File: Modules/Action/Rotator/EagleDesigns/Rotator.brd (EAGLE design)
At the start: 100 x 80 mm, 9 parts, among them U2 ATMEGA328P_TQFP

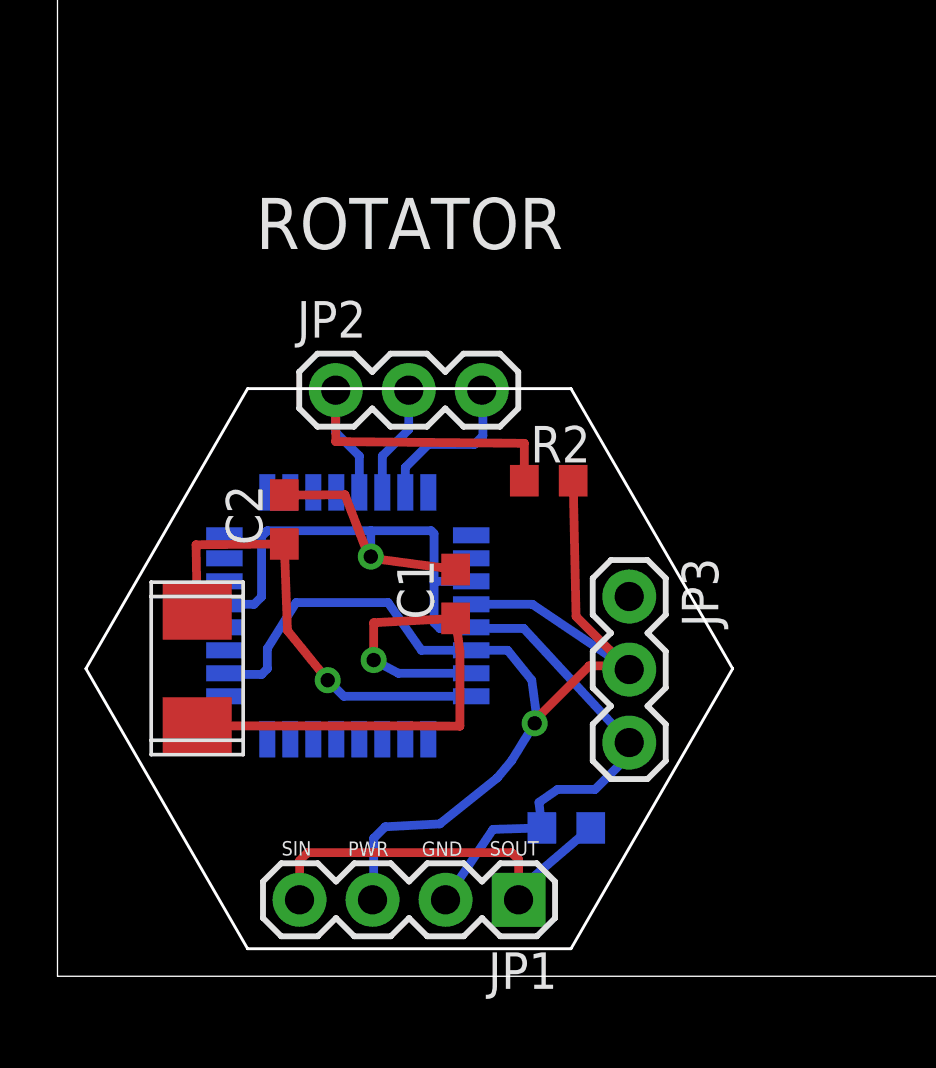
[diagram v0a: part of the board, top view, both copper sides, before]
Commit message: Revert "Merge branch 'version-1.2'"
This reverts commit 982d9c85d5bd00c48b539e840003de48d3cf178d, reversing
changes made to b3895ae538c161df72313035d3e956c7a5ec4dbc.
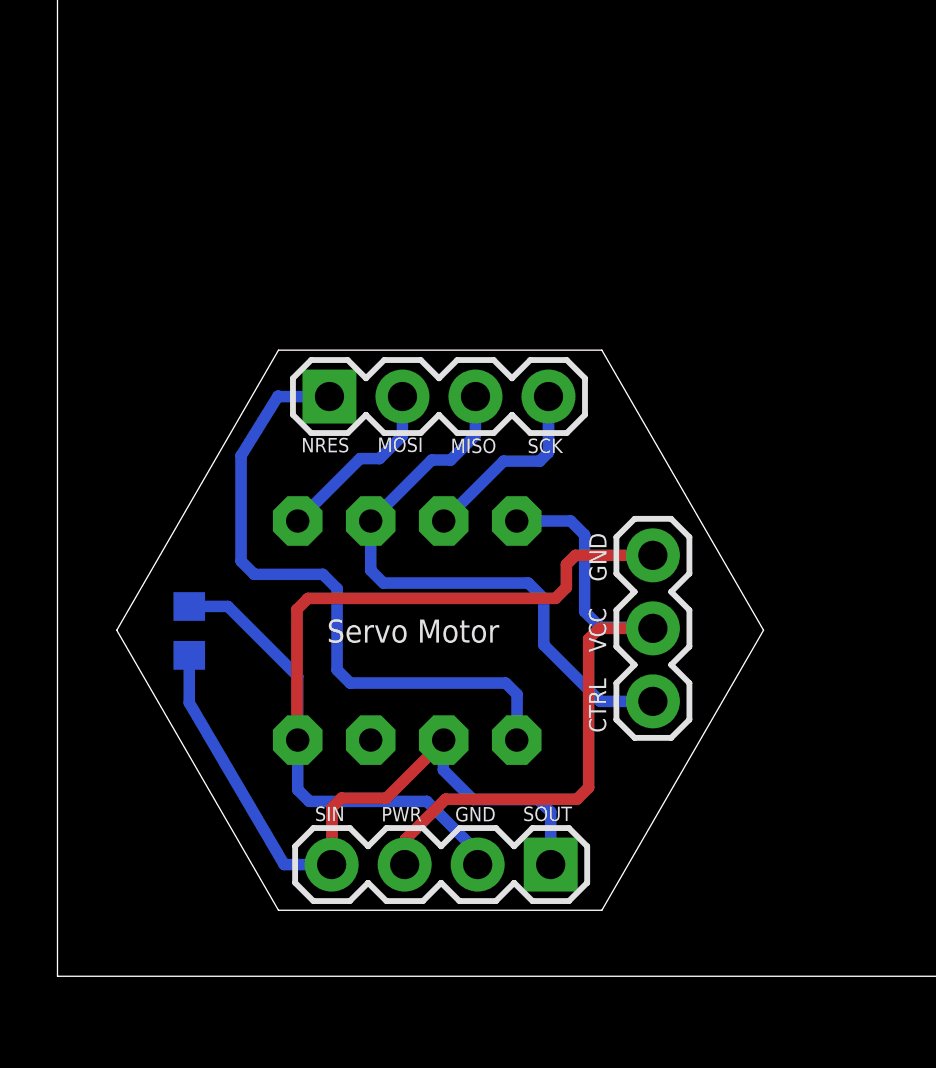
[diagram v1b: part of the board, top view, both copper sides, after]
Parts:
- removed C1, C2: 22pF, adafruit:C0603
- removed R2: 10K, resistor:R0603
- removed U$2: NX503, MakerWear:NX503
- removed U2: ATMEGA328P_TQFP, SparkFun-DigitalIC:TQFP32-08
- added U1: TINY85-20-DIP, SparkFun-DigitalIC:DIP08
- JP2: device SparkFun-Connectors:1X03 -> SparkFun-Connectors:1X04
- moved R1 14.8 mm to (4.58, 12.0), turned to 270 degrees
- moved JP3 3.74 mm to (20.7, 9.56), turned to 90 degrees
- moved JP1 1.66 mm to (17.2, 3.89)
- moved JP2 0.31 mm to (9.46, 20.2)
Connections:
- removed net 1X3SIN: U2.23
- removed net N$1: C1.1, U$2.P$1, U2.7
- removed net N$3: C2.1, U$2.P$2, U2.8
- removed net RESET: JP2.1, R2.1, U2.29
- removed net RX: JP2.2, U2.30
- removed net TX: JP2.3, U2.31
- new net MOSI: JP2.2, U1.5
- new net NRES: JP2.1, U1.1
- new net OUT(MISO): JP2.3, JP3.1, U1.6
- new net SCK: JP2.4, U1.7
- net 1X3SIN-SOUT: now also U1.2
- net GND: now also U1.4; no longer C1.2, C2.2, U2.21, U2.3, U2.5
- net VCC: now also U1.8; no longer R2.2, U2.18, U2.4, U2.6
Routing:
- net NRES: track 0.00 -> 22.7 mm
- net OUT(MISO): track 0.00 -> 20.6 mm
- net N$1: track 20.6 -> 0.00 mm, vias 1 -> 0
- net VCC: track 43.5 -> 23.4 mm, vias 1 -> 0
- net N$3: track 15.8 -> 0.00 mm, vias 1 -> 0
- net RESET: track 13.5 -> 0.00 mm
- net 1X3SIN-SOUT: track 14.4 -> 23.9 mm
- net SCK: track 0.00 -> 6.58 mm
- net GND: track 40.9 -> 34.5 mm, vias 1 -> 0
- net MOSI: track 0.00 -> 6.23 mm
- net TX: track 5.62 -> 0.00 mm
- net RX: track 3.94 -> 0.00 mm
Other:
- outline, holes or cut-outs redrawn
- board text added: "CTRL"
- board text added: "MISO"
- board text added: "MOSI"
- board text added: "MW-V3"
- board text added: "NRES"
- board text added: "SCK"
- board text added: "Servo Motor"
- board text added: "VCC"
- board text removed: "ROTATOR"

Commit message: added Rotator #30 eagle files
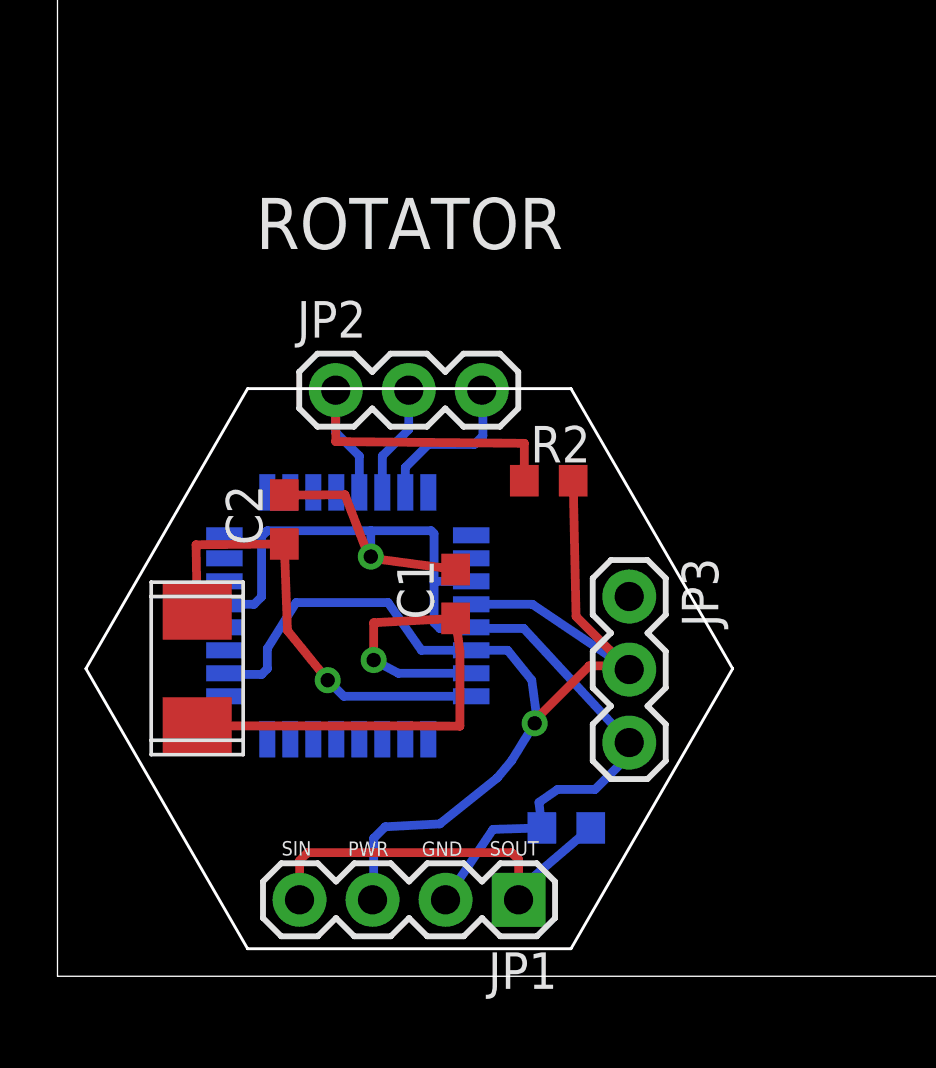
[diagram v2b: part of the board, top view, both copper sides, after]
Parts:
- removed U1: TINY85-20-DIP, SparkFun-DigitalIC:DIP08
- added C1, C2: 22pF, adafruit:C0603
- added R2: 10K, resistor:R0603
- added U$2: NX503, MakerWear:NX503
- added U2: ATMEGA328P_TQFP, SparkFun-DigitalIC:TQFP32-08
- JP2: device SparkFun-Connectors:1X04 -> SparkFun-Connectors:1X03
- moved R1 14.8 mm to (17.7, 5.16), turned to 180 degrees
- moved JP3 3.74 mm to (19.9, 13.2), turned to 270 degrees
- moved JP1 1.66 mm to (16.0, 2.66)
- moved JP2 0.31 mm to (9.68, 20.4)
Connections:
- removed net MOSI: JP2.2, U1.5
- removed net NRES: JP2.1, U1.1
- removed net OUT(MISO): JP2.3, JP3.1, U1.6
- removed net SCK: JP2.4, U1.7
- new net 1X3SIN: U2.23
- new net N$1: C1.1, U$2.P$1, U2.7
- new net N$3: C2.1, U$2.P$2, U2.8
- new net RESET: JP2.1, R2.1, U2.29
- new net RX: JP2.2, U2.30
- new net TX: JP2.3, U2.31
- net 1X3SIN-SOUT: no longer U1.2
- net GND: now also C1.2, C2.2, U2.21, U2.3, U2.5; no longer U1.4
- net VCC: now also R2.2, U2.18, U2.4, U2.6; no longer U1.8
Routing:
- net NRES: track 22.7 -> 0.00 mm
- net OUT(MISO): track 20.6 -> 0.00 mm
- net N$1: track 0.00 -> 20.6 mm, vias 0 -> 1
- net VCC: track 23.4 -> 43.5 mm, vias 0 -> 1
- net N$3: track 0.00 -> 15.8 mm, vias 0 -> 1
- net RESET: track 0.00 -> 13.5 mm
- net 1X3SIN-SOUT: track 23.9 -> 14.4 mm
- net SCK: track 6.58 -> 0.00 mm
- net GND: track 34.5 -> 40.9 mm, vias 0 -> 1
- net MOSI: track 6.23 -> 0.00 mm
- net TX: track 0.00 -> 5.62 mm
- net RX: track 0.00 -> 3.94 mm
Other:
- outline, holes or cut-outs redrawn
- board text added: "ROTATOR"
- board text removed: "CTRL"
- board text removed: "MISO"
- board text removed: "MOSI"
- board text removed: "MW-V3"
- board text removed: "NRES"
- board text removed: "SCK"
- board text removed: "Servo Motor"
- board text removed: "VCC"
